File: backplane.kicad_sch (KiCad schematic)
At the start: 2 parts, among them J200 09031967921, U200 PESD5V0S2BT

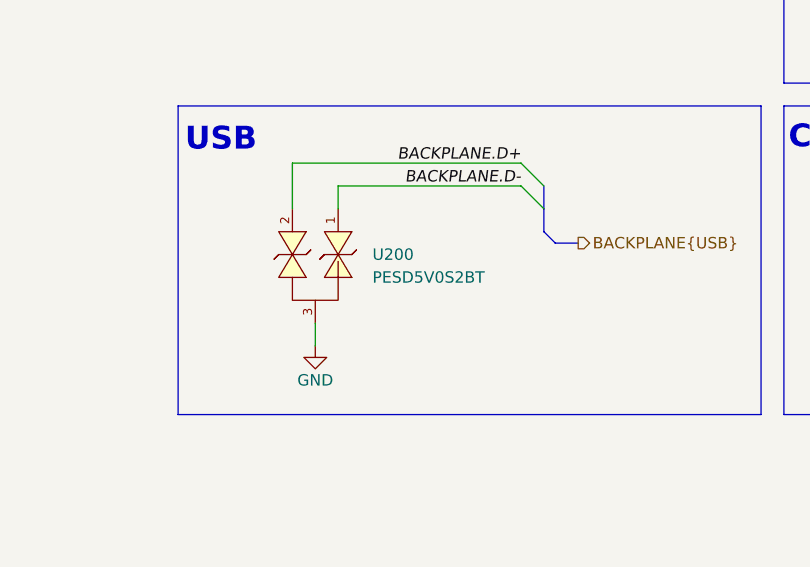
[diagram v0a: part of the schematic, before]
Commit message: [#12] Change USB TVS
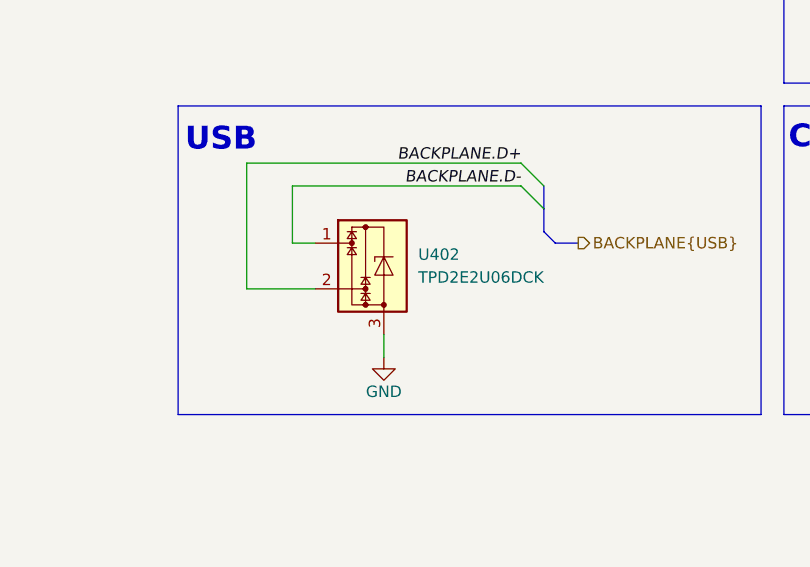
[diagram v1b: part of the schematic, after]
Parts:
- removed U200: PESD5V0S2BT, Package_TO_SOT_SMD:SOT-23, symbol PESD5V0S2BT:PESD5V0S2BT
- added U402: TPD2E2U06DCK, Package_TO_SOT_SMD:SOT-323_SC-70, symbol Power_Protection:TPD2E2U06DCK
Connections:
- net BACKPLANE.D+: now also U402.2
- net BACKPLANE.D-: now also U402.1
- net GND: now also U402.3
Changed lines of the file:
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@@
 	(wire
 		(pts
+			(xy 193.04 147.32) (xy 185.42 147.32)
+		)
+		(stroke
+			(width 0)
+			(type default)
+		)
+	)
+	(wire
+		(pts
 			(xy 91.44 182.88) (xy 41.91 182.88)
 		)
@@
 	(wire
 		(pts
-			(xy 190.5 133.35) (xy 190.5 138.43)
+			(xy 185.42 133.35) (xy 185.42 147.32)
 		)
 		(stroke
@@
 	(wire
 		(pts
-			(xy 195.58 135.89) (xy 215.9 135.89)
+			(xy 190.5 135.89) (xy 215.9 135.89)
 		)
 		(stroke
@@
 	(wire
 		(pts
-			(xy 193.04 151.13) (xy 193.04 153.67)
+			(xy 200.66 152.4) (xy 200.66 154.94)
 		)
 		(stroke
@@
 	(wire
 		(pts
-			(xy 195.58 135.89) (xy 195.58 138.43)
+			(xy 190.5 135.89) (xy 190.5 142.24)
 		)
 		(stroke
@@
 	(wire
 		(pts
-			(xy 190.5 133.35) (xy 215.9 133.35)
+			(xy 185.42 133.35) (xy 215.9 133.35)
 		)
 		(stroke
@@
 	(wire
 		(pts
+			(xy 190.5 142.24) (xy 193.04 142.24)
+		)
+		(stroke
+			(width 0)
+			(type default)
+		)
+	)
+	(wire
+		(pts
 			(xy 53.34 35.56) (xy 91.44 35.56)
 		)
@@
 	)
 	(symbol
+		(lib_id "Power_Protection:TPD2E2U06DCK")
+		(at 200.66 144.78 0)
+		(unit 1)
+		(exclude_from_sim no)
+		(in_bom yes)
+		(on_board yes)
+		(dnp no)
+		(fields_autoplaced yes)
+		(property "Reference" "U402"
+			(at 204.47 143.5099 0)
+			(effects
+				(font
+					(size 1.27 1.27)
+				)
+				(justify left)
+			)
+		)
+		(property "Value" "TPD2E2U06DCK"
+			(at 204.47 146.0499 0)
+			(effects
+				(font
+					(size 1.27 1.27)
+				)
+				(justify left)
+			)
+		)
+		(property "Footprint" "Package_TO_SOT_SMD:SOT-323_SC-70"
+			(at 180.34 151.13 0)
+			(effects
+				(font
+					(size 1.27 1.27)
+				)
+				(hide yes)
+			)
+		)
+		(property "Datasheet" "http://www.ti.com/lit/ds/symlink/tpd2e2u06.pdf"
+			(at 195.58 139.7 0)
+			(effects
+				(font
+					(size 1.27 1.27)
+				)
+				(hide yes)
+			)
+		)
+		(property "Description" "Dual-Channel High-Speed ESD Protection, SC-70"
+			(at 200.66 144.78 0)
+			(effects
+				(font
+					(size 1.27 1.27)
+				)
+				(hide yes)
+			)
+		)
+		(pin "2"
+		)
+		(pin "1"
+		)
+		(pin "3"
+		)
+		(instances
+			(project "base-module"
+				(path "/090a8e41-87a8-4fb1-998b-60a2c0dc4cee/ff3476d7-2f10-4f79-9864-988601c7ce1b"
+					(reference "U402")
+					(unit 1)
+				)
+			)
+		)
+	)
+	(symbol
 		(lib_id "power:GND")
 		(at 78.74 45.72 270)
@@
 		(lib_name "GND_1")
 		(lib_id "power:GND")
-		(at 193.04 153.67 0)
+		(at 200.66 154.94 0)
 		(unit 1)
 		(exclude_from_sim no)
@@
 		(dnp no)
 		(property "Reference" "#PWR0235"
-			(at 193.04 160.02 0)
+			(at 200.66 161.29 0)
 			(effects
 				(font
@@
 		)
 		(property "Value" "GND"
-			(at 193.04 157.48 0)
+			(at 200.66 158.75 0)
 			(effects
 				(font
@@
 		)
 		(property "Footprint" ""
-			(at 193.04 153.67 0)
+			(at 200.66 154.94 0)
 			(effects
 				(font
@@
 		)
 		(property "Datasheet" ""
-			(at 193.04 153.67 0)
+			(at 200.66 154.94 0)
 			(effects
 				(font
@@
 		)
 		(property "Description" "Power symbol creates a global label with name \"GND\" , ground"
-			(at 193.04 153.67 0)
+			(at 200.66 154.94 0)
 			(effects
 				(font
@@
 					(unit 1)
 				)
-			)
-		)
-	)
-	(symbol
-		(lib_id "PESD5V0S2BT:PESD5V0S2BT")
-		(at 193.04 146.05 180)
-		(unit 1)
-		(exclude_from_sim no)
-		(in_bom yes)
-		(on_board yes)
-		(dnp no)
-		(fields_autoplaced yes)
-		(property "Reference" "U200"
-			(at 199.39 143.5099 0)
-			(effects
-				(font
-					(size 1.27 1.27)
-				)
-				(justify right)
-			)
-		)
-		(property "Value" "PESD5V0S2BT"
-			(at 199.39 146.0499 0)
-			(effects
-				(font
-					(size 1.27 1.27)
-				)
-				(justify right)
-			)
-		)
-		(property "Footprint" "Package_TO_SOT_SMD:SOT-23"
-			(at 193.04 146.05 0)
-			(effects
-				(font
-					(size 1.27 1.27)
-				)
-				(hide yes)
-			)
-		)
-		(property "Datasheet" "https://www.lcsc.com/datasheet/lcsc_datasheet_2501101716_HXY-MOSFET-PESD5V0S2BT_C5451656.pdf"
-			(at 193.04 146.05 0)
-			(effects
-				(font
-					(size 1.27 1.27)
-				)
-				(hide yes)
-			)
-		)
-		(property "Description" "11A 8V 8V Bidirectional 5V SOT-23 ESD and Surge Protection (TVS/ESD)"
-			(at 193.04 146.05 0)
-			(effects
-				(font
-					(size 1.27 1.27)
-				)
-				(hide yes)
-			)
-		)
-		(pin "3"
-		)
-		(pin "1"
-		)
-		(pin "2"
-		)
-		(instances
-			(project ""
-				(path "/090a8e41-87a8-4fb1-998b-60a2c0dc4cee/ff3476d7-2f10-4f79-9864-988601c7ce1b"
-					(reference "U200")
-					(unit 1)
-				)
